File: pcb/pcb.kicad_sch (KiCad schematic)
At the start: 4 parts, among them J1 Botones, J2 Pedales+Velocimetro+Monedas, J3 Volante

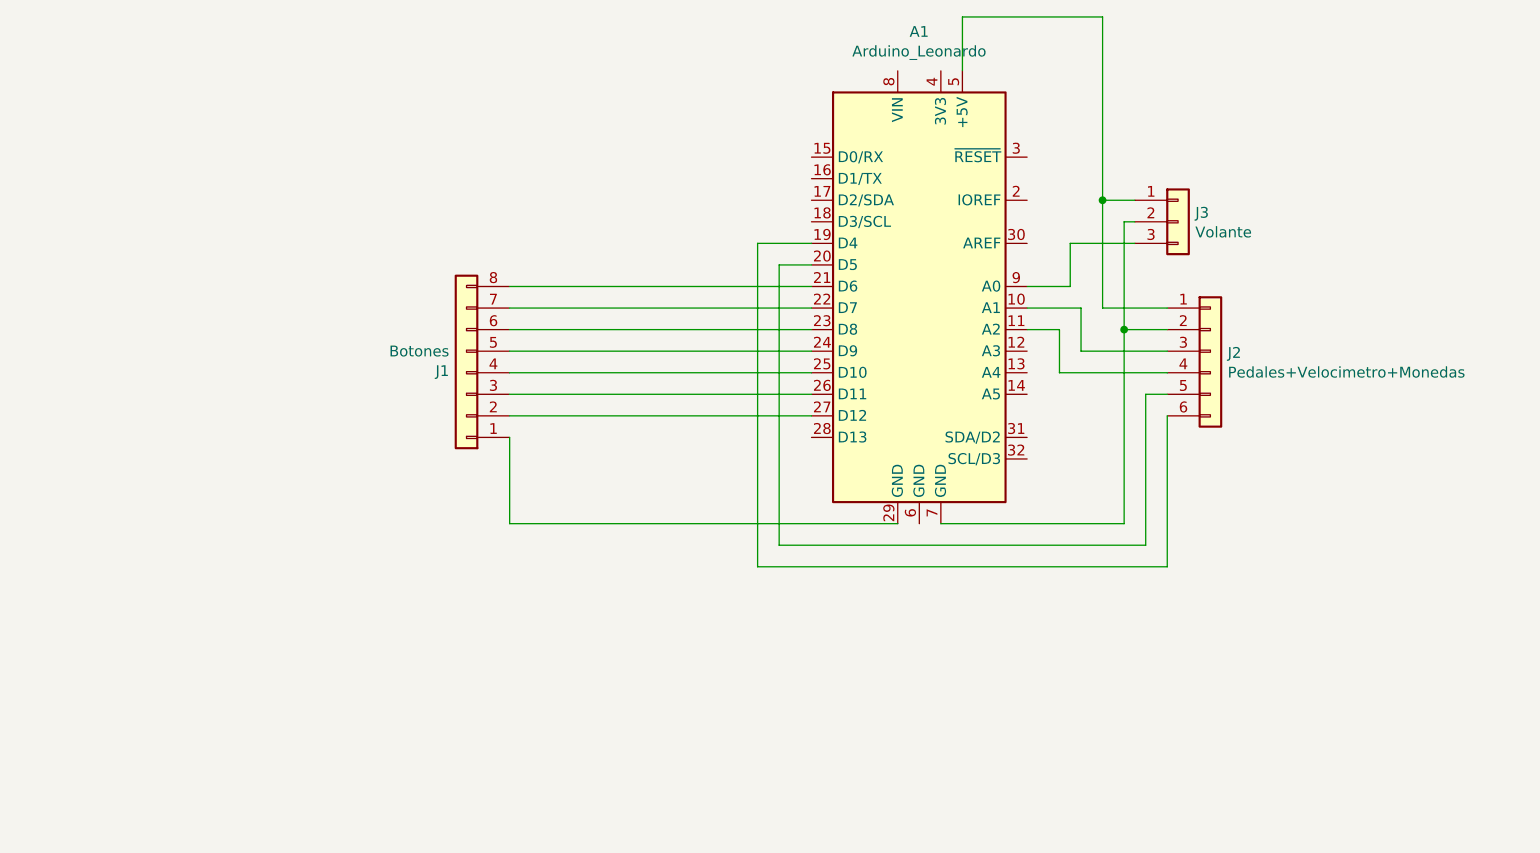
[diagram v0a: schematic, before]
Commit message: Add layout and schematic prints
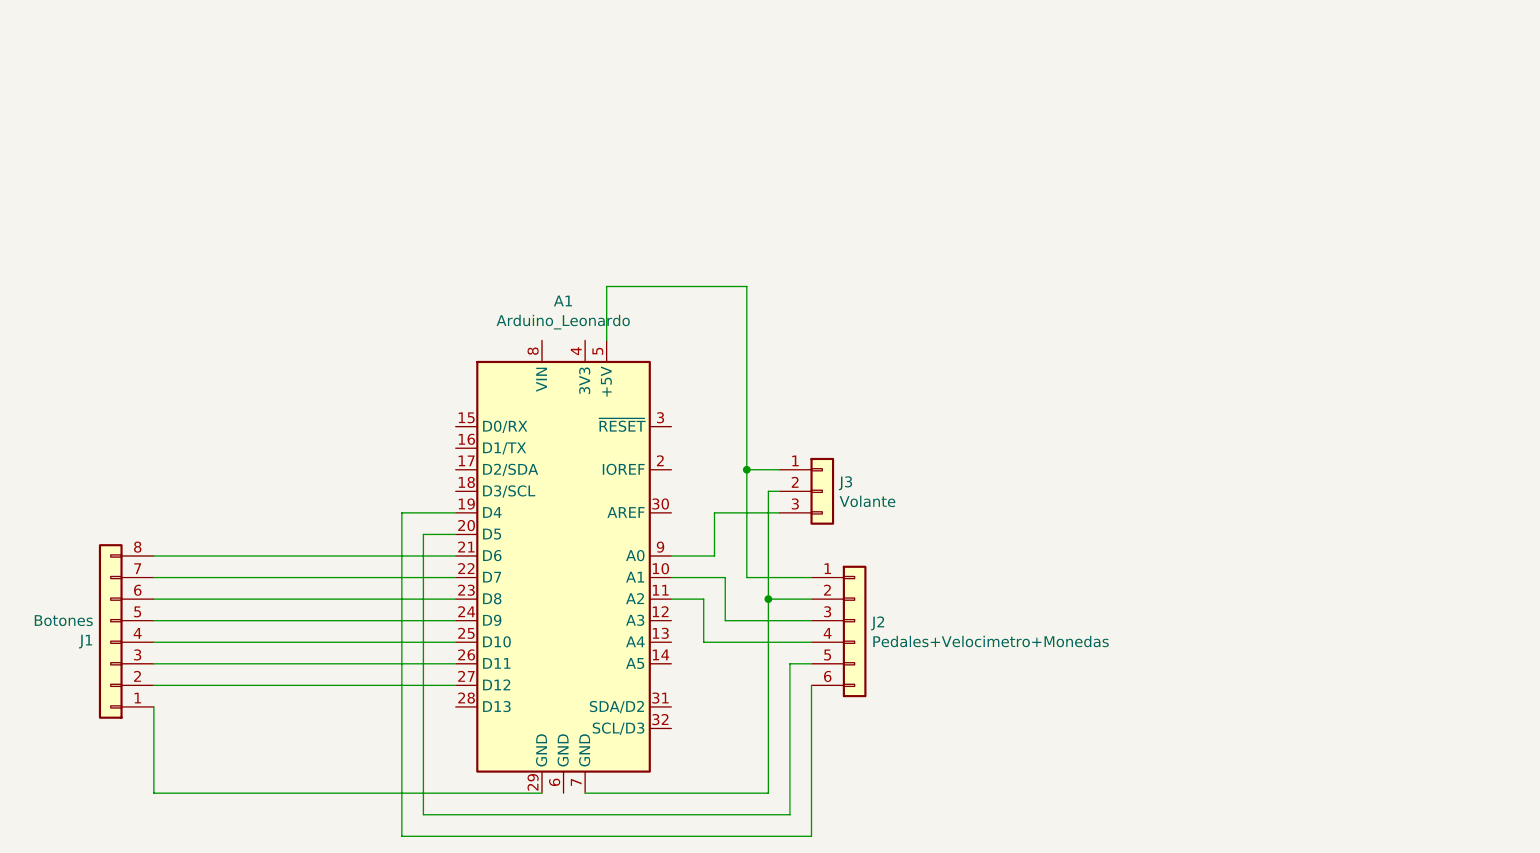
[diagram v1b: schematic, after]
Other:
- title: (none) -> Ches Pur Ofi
- moved on the sheet: A1, J1, J2, J3
